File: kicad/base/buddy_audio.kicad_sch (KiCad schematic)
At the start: 14 parts, among them U3 ICE40UP5K-SG48ITR, U4 AP2127K-1.2, U5 W25Q32JVSS

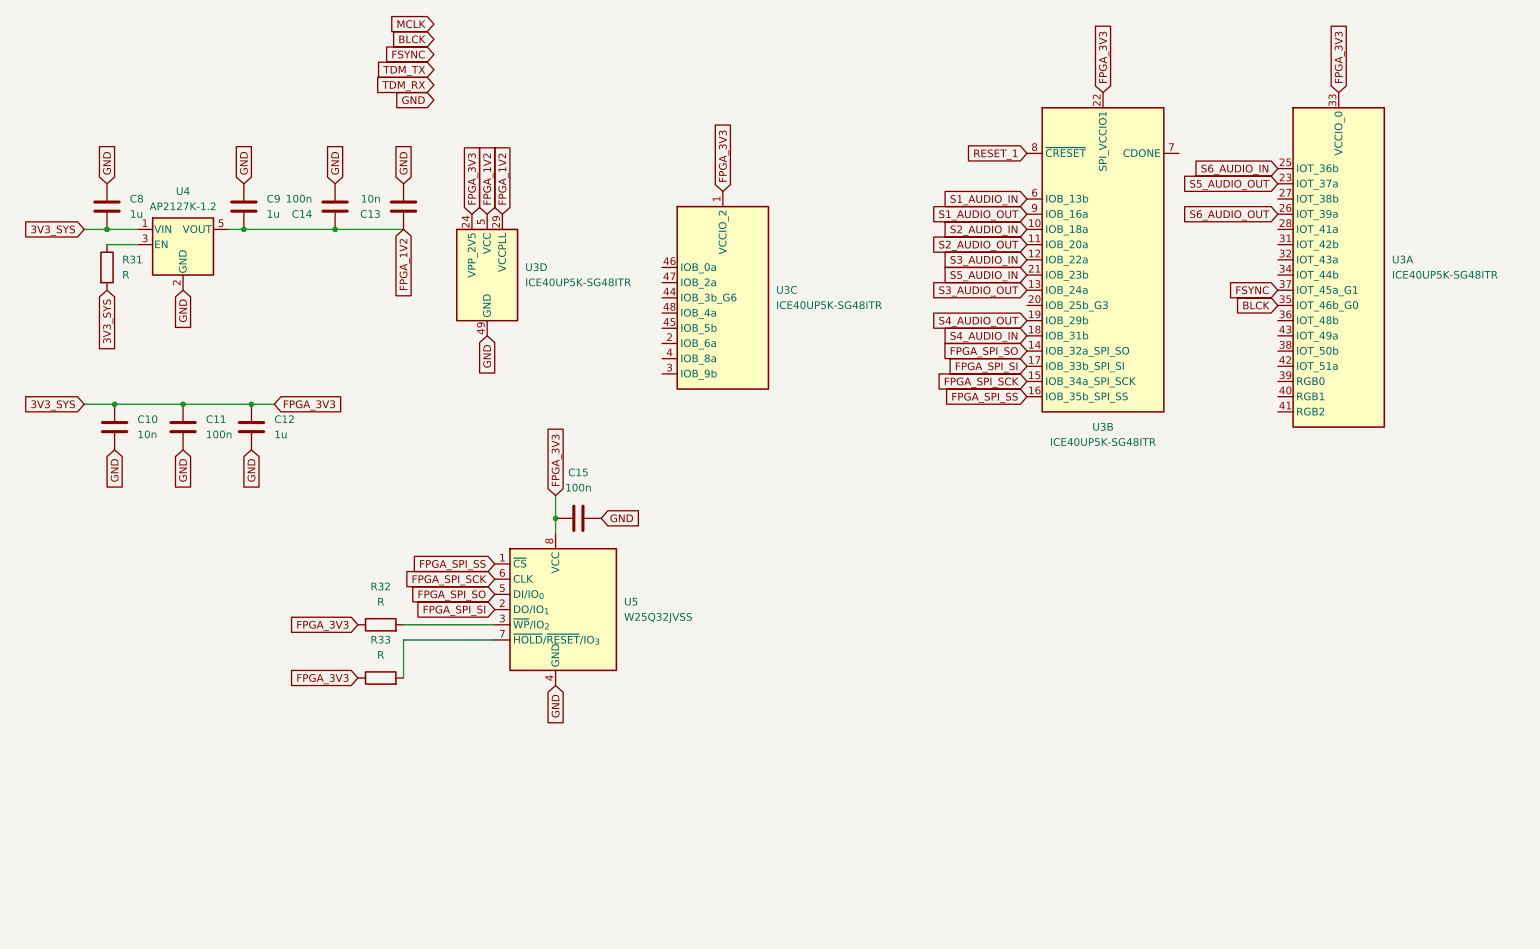
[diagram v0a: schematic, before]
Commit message: Add new brains
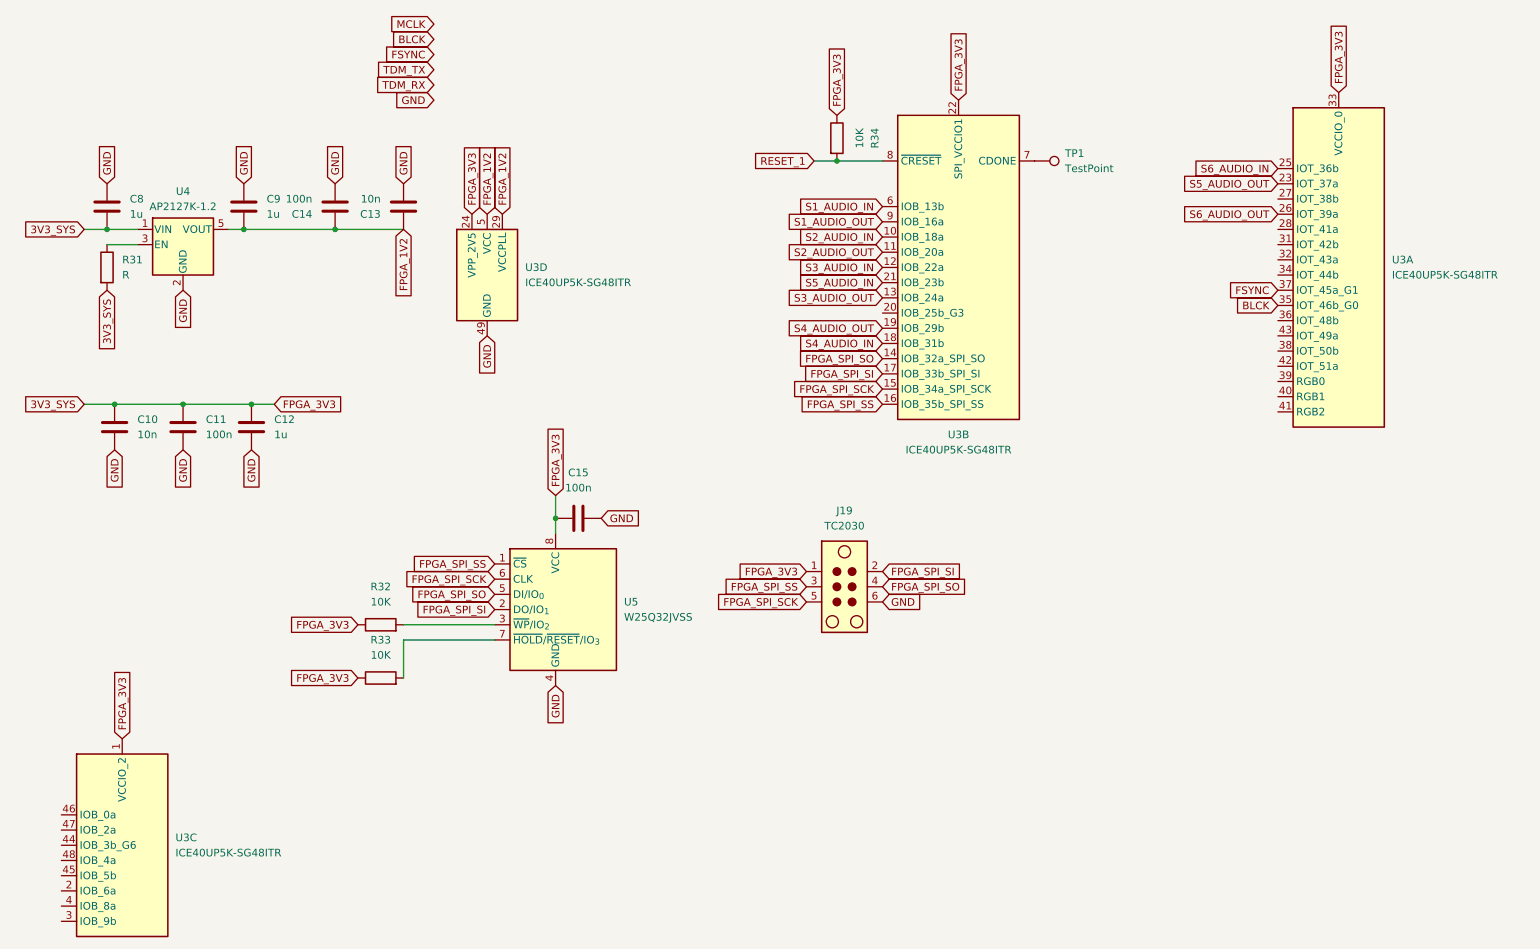
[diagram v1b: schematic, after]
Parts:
- added J19: TC2030, Connector:Tag-Connect_TC2030-IDC-NL_2x03_P1.27mm_Vertical, symbol Connector:TC2030
- added R34: 10K, Resistor_SMD:R_0603_1608Metric, symbol Device:R
- added TP1: TestPoint, TestPoint:TestPoint_THTPad_D1.0mm_Drill0.5mm, symbol Connector:TestPoint
- R32, R33: value R -> 10K
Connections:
- net 3V3_SYS: now also J19.1, R34.1
- net FPGA_SPI_SCK: now also J19.5
- net FPGA_SPI_SI: now also J19.2
- net FPGA_SPI_SO: now also J19.4
- net FPGA_SPI_SS: now also J19.3
- net GND: now also J19.6
- net RESET_1: now also R34.2
- net at U3.7 (CDONE): now also TP1.1
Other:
- moved on the sheet: U3B, U3C
